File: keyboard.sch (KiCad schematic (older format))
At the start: 80 parts

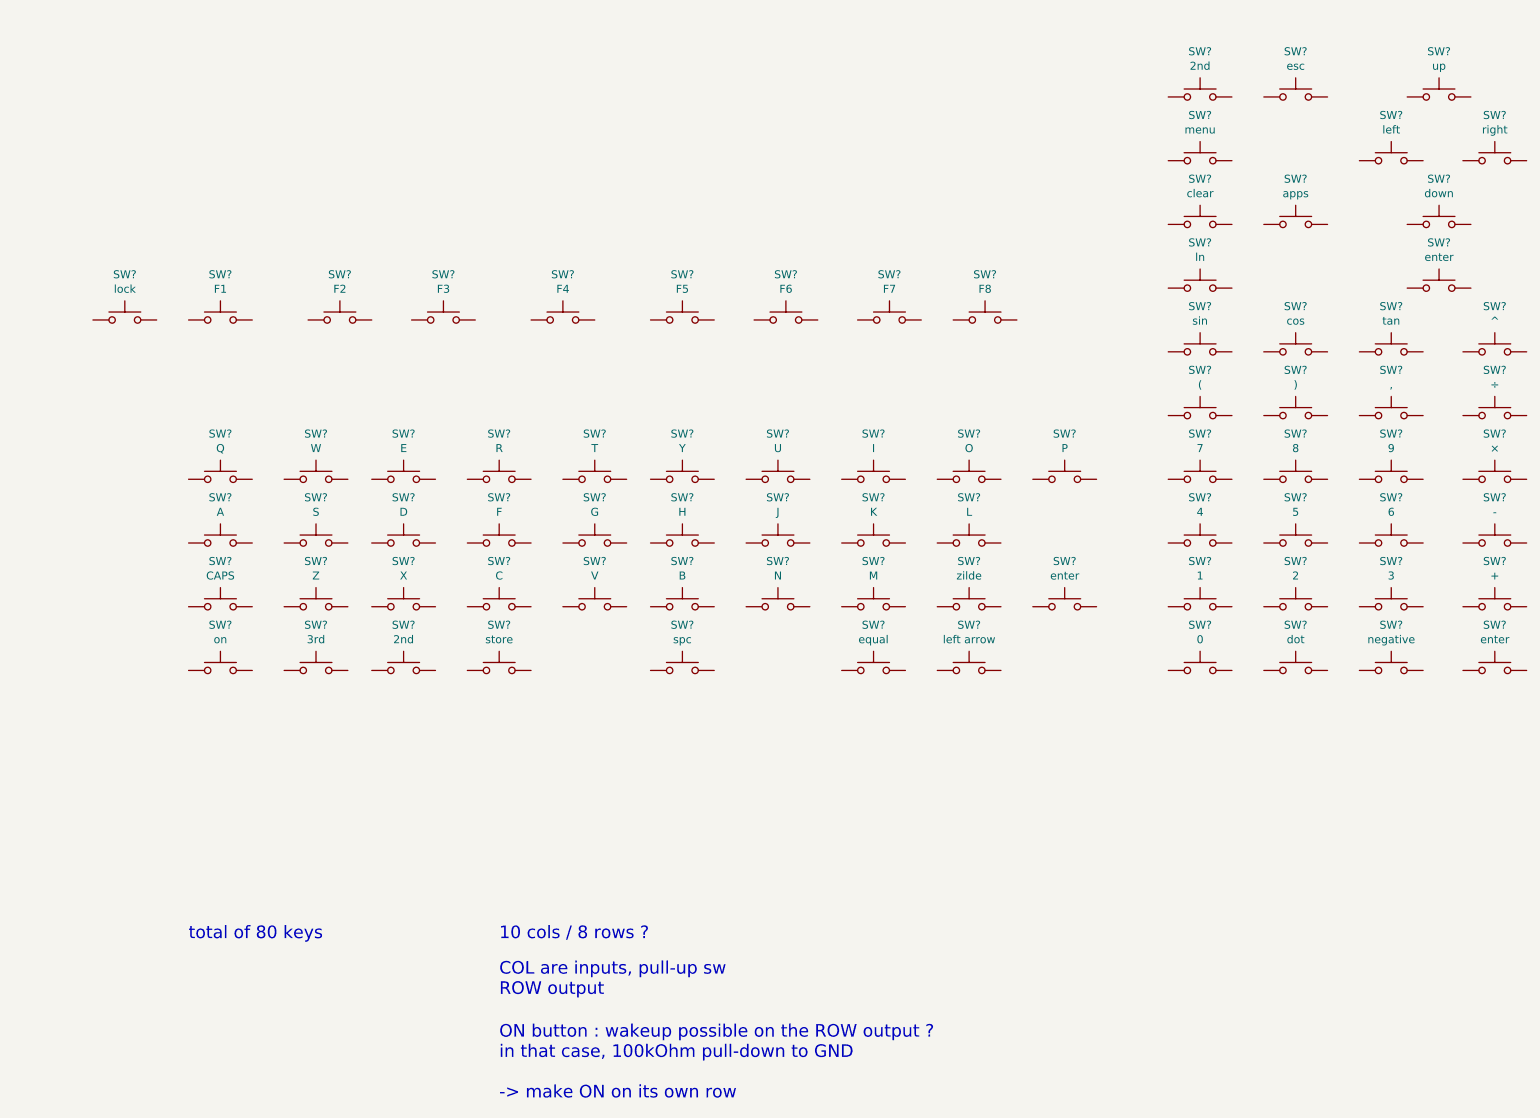
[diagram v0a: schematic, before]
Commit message: Switch to STM32, wire stuff
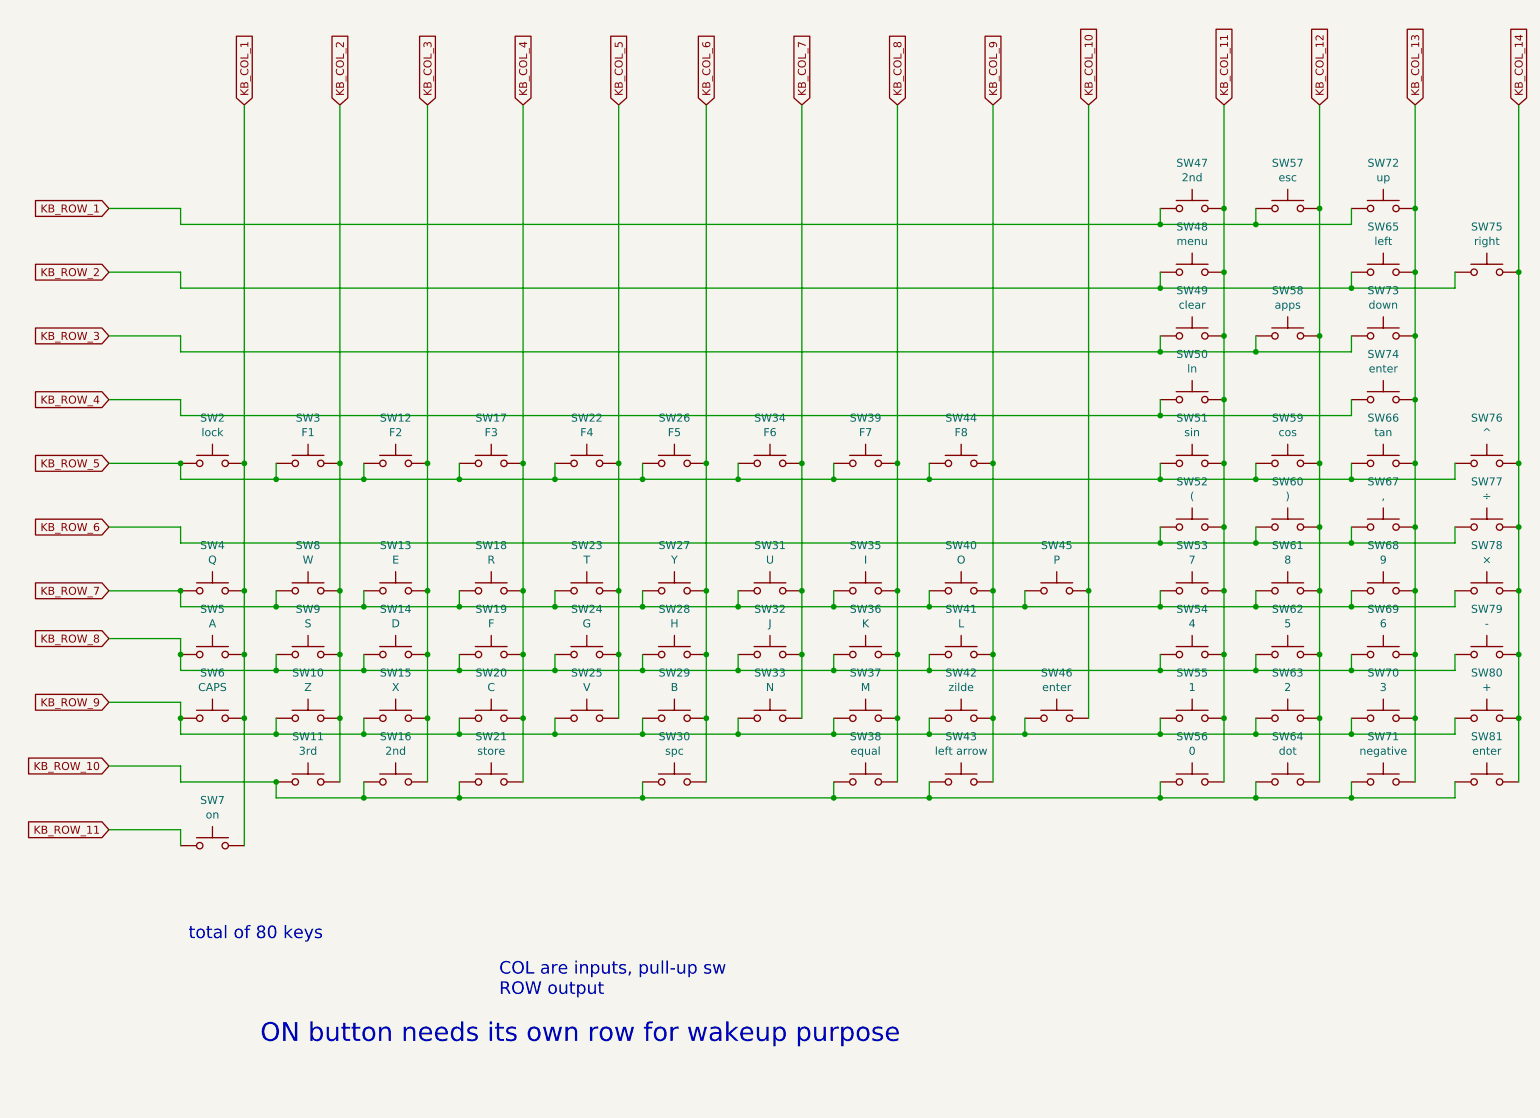
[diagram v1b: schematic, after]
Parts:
- gave numbers to parts that had none: 80
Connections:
- net KB_ROW_5: now reaches SW3.1
- net KB_ROW_5: now also SW12.1, SW17.1, SW2.1, SW22.1, SW26.1, SW34.1, SW39.1, SW44.1, SW51.1, SW59.1, SW66.1, SW76.1
- net KB_COL_2: now reaches SW3.2
- net KB_COL_2: now also SW10.2, SW11.2, SW8.2, SW9.2
- net KB_COL_3: now reaches SW12.2
- net KB_COL_3: now also SW13.2, SW14.2, SW15.2, SW16.2
- net KB_COL_4: now reaches SW17.2
- net KB_COL_4: now also SW18.2, SW19.2, SW20.2, SW21.2
- net KB_COL_5: now reaches SW22.2
- net KB_COL_5: now also SW23.2, SW24.2, SW25.2
- net KB_COL_6: now reaches SW26.2
- net KB_COL_6: now also SW27.2, SW28.2, SW29.2, SW30.2
- net KB_COL_7: now reaches SW34.2
- net KB_COL_7: now also SW31.2, SW32.2, SW33.2
- net KB_COL_8: now reaches SW39.2
- net KB_COL_8: now also SW35.2, SW36.2, SW37.2, SW38.2
- net KB_COL_9: now reaches SW44.2
- net KB_COL_9: now also SW40.2, SW41.2, SW42.2, SW43.2
- net KB_ROW_7: now reaches SW4.1
- net KB_ROW_7: now also SW13.1, SW18.1, SW23.1, SW27.1, SW31.1, SW35.1, SW40.1, SW45.1, SW53.1, SW61.1, SW68.1, SW78.1, SW8.1
- net KB_COL_1: now reaches SW4.2
- net KB_COL_1: now also SW2.2, SW5.2, SW6.2, SW7.2
- net KB_COL_10: now reaches SW45.2
- net KB_COL_10: now also SW46.2
- net KB_ROW_8: now reaches SW5.1
- net KB_ROW_8: now also SW14.1, SW19.1, SW24.1, SW28.1, SW32.1, SW36.1, SW41.1, SW54.1, SW62.1, SW69.1, SW79.1, SW9.1
- net KB_ROW_9: now reaches SW6.1
- net KB_ROW_9: now also SW10.1, SW15.1, SW20.1, SW25.1, SW29.1, SW33.1, SW37.1, SW42.1, SW46.1, SW55.1, SW63.1, SW70.1, SW80.1
- net KB_ROW_11: now reaches SW7.1
- net KB_ROW_10: now reaches SW11.1
- net KB_ROW_10: now also SW16.1, SW21.1, SW30.1, SW38.1, SW43.1, SW56.1, SW64.1, SW71.1, SW81.1
- net KB_COL_11: now reaches SW56.2
- net KB_COL_11: now also SW47.2, SW48.2, SW49.2, SW50.2, SW51.2, SW52.2, SW53.2, SW54.2, SW55.2
- net KB_COL_12: now reaches SW64.2
- net KB_COL_12: now also SW57.2, SW58.2, SW59.2, SW60.2, SW61.2, SW62.2, SW63.2
- net KB_COL_13: now reaches SW71.2
- net KB_COL_13: now also SW65.2, SW66.2, SW67.2, SW68.2, SW69.2, SW70.2, SW72.2, SW73.2, SW74.2
- net KB_COL_14: now reaches SW81.2
- net KB_COL_14: now also SW75.2, SW76.2, SW77.2, SW78.2, SW79.2, SW80.2
- net KB_ROW_6: now reaches SW52.1
- net KB_ROW_6: now also SW60.1, SW67.1, SW77.1
- net KB_ROW_4: now reaches SW50.1
- net KB_ROW_4: now also SW74.1
- net KB_ROW_3: now reaches SW49.1
- net KB_ROW_3: now also SW58.1, SW73.1
- net KB_ROW_2: now reaches SW75.1
- net KB_ROW_2: now also SW48.1, SW65.1
- net KB_ROW_1: now reaches SW57.1
- net KB_ROW_1: now also SW47.1, SW72.1
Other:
- note added: "ON button needs its own row for wakeup purpose"
- note removed: "10 cols / 8 rows ?"
- note removed: "ON button : wakeup possible on the ROW output ?\nin that case, 100kOhm pull-down to GND\n\n-> make ON on its own row"
- moved on the sheet: SW10, SW11, SW12, SW13, SW14, SW15, SW16, SW17, SW18, SW19, SW2, SW20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
